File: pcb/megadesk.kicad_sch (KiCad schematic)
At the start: 25 parts, among them J1 Interface, J2 FFC, J3 AVR-ISP-6, U1 7812, U2 HT7550-1, U3 ATtiny841-SS, U4 MCP2003B

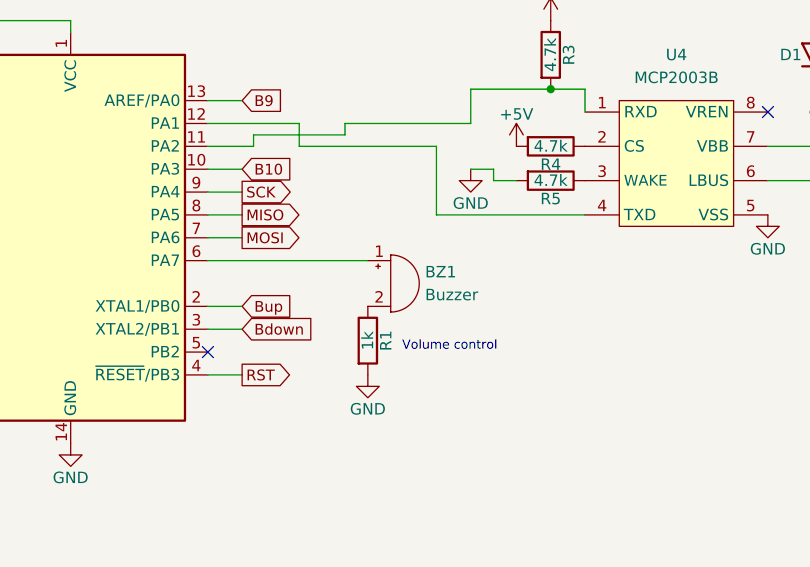
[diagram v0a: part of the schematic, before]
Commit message: kicad v7
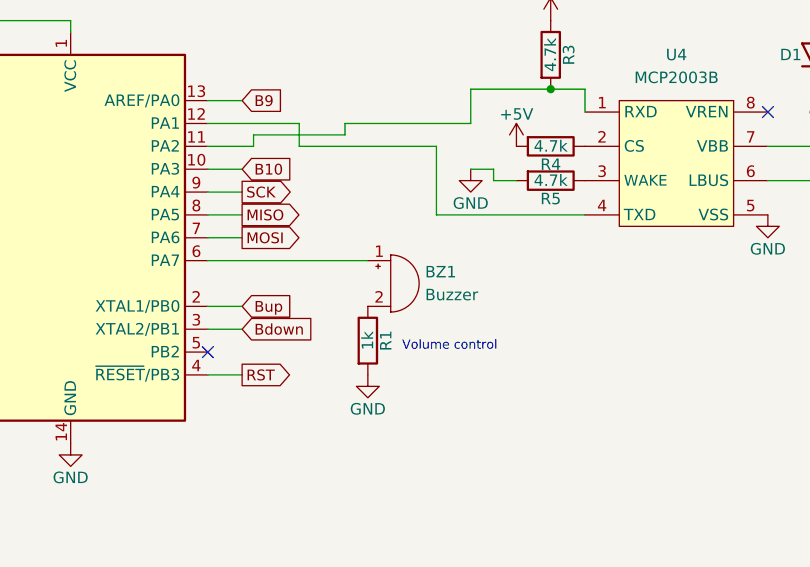
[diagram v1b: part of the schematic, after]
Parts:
- U2: symbol Regulator_Linear:MCP1700-2502E_SOT89 -> Regulator_Linear:MCP1700x-120xxMB
